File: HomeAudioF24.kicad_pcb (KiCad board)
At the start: 4 copper layers, 214 x 114 mm, 26 parts, among them U1 LF356M, U2 LF356M, U3 LF356M, U4 LF356M, U5 LF356M, U6 LF356M, U7 LF356M

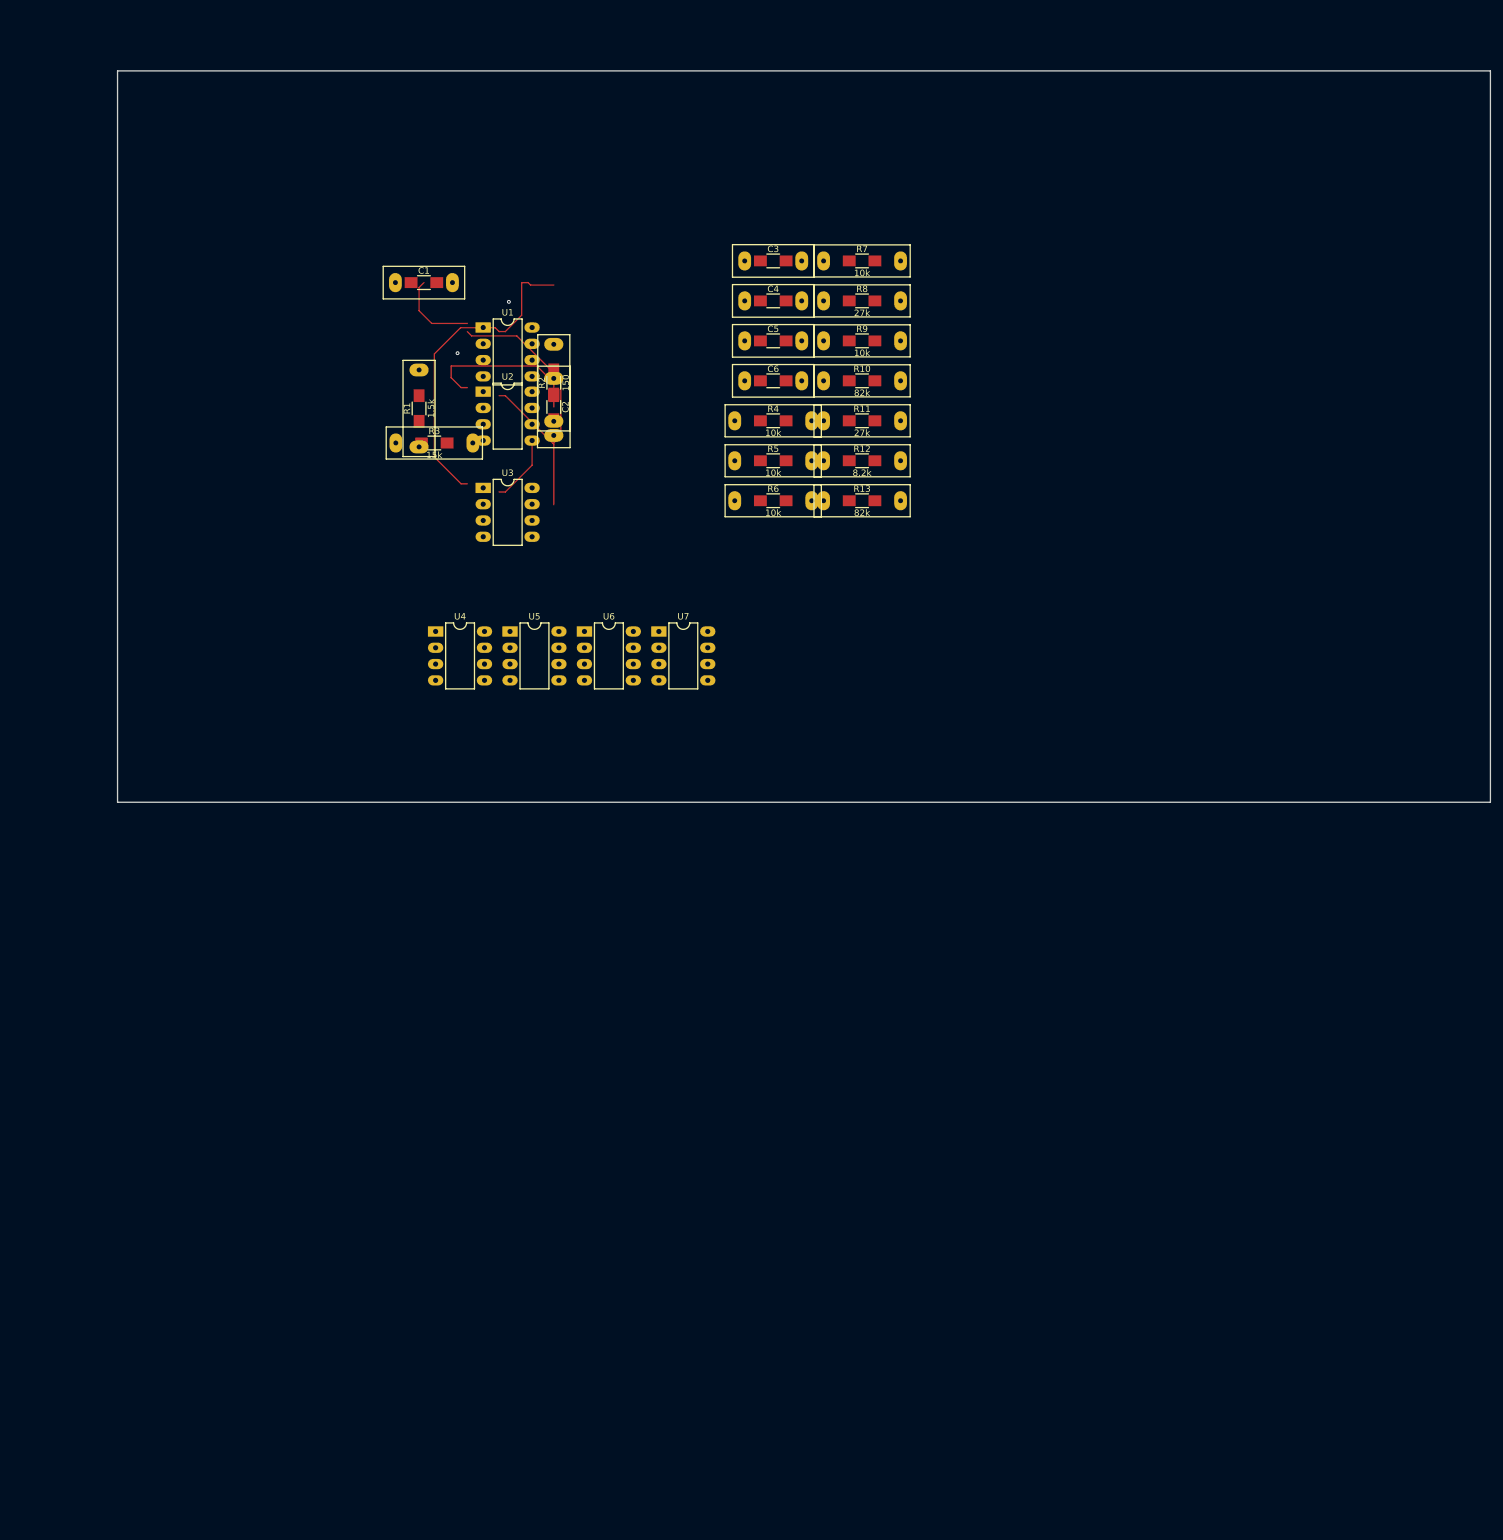
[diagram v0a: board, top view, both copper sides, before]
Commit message: First Major Revision
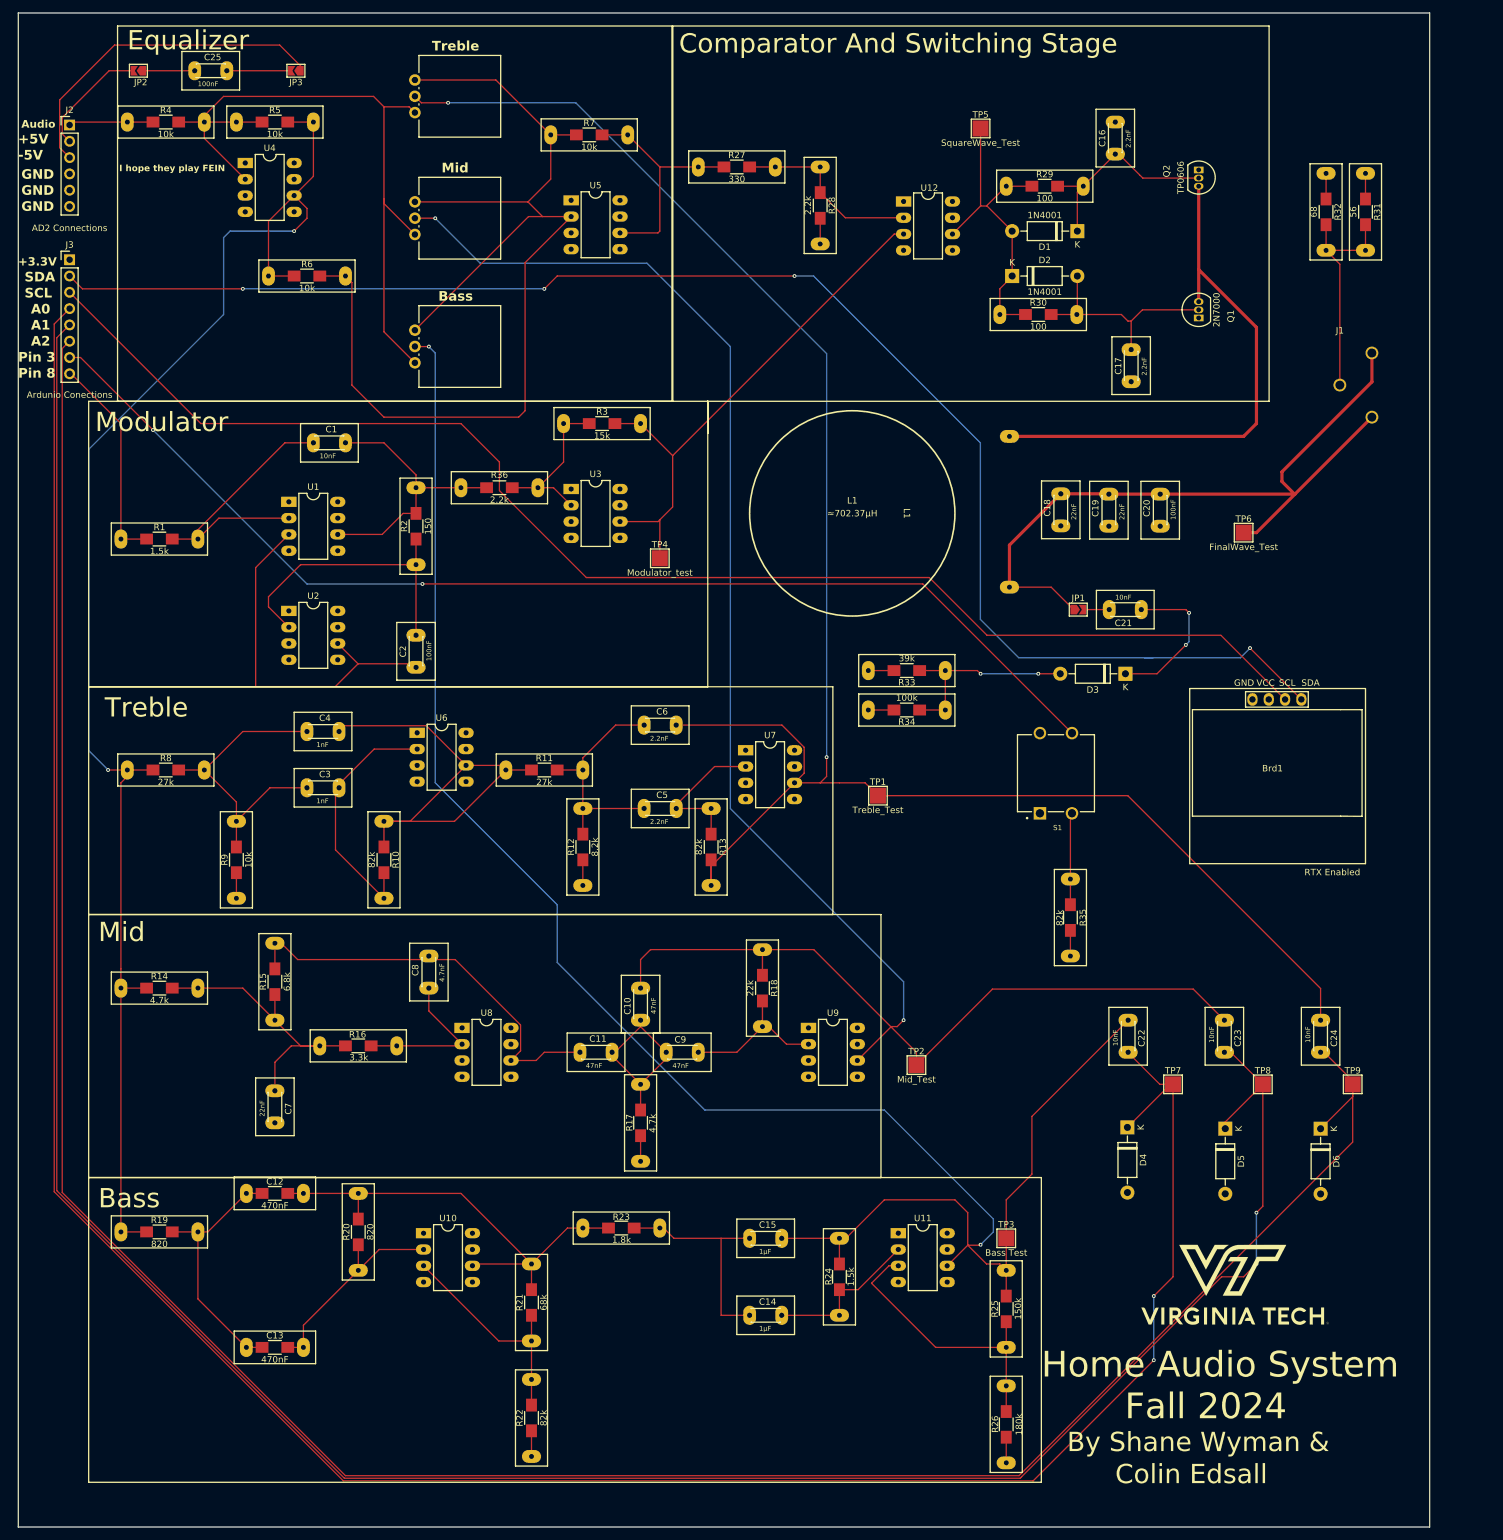
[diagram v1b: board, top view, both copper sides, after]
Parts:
- added Brd1: SSD1306, Display_New:128x64OLED SSD1306, F.Cu at (215.5, 142.6)
- added C10: 47nF, ColorOrgan:C_Disc_D4.3mm_W1.9mm_P5.00mm_Handsolder, F.Cu at (116.5, 177.0)
- added C11: 47nF, ColorOrgan:C_Disc_D4.3mm_W1.9mm_P5.00mm_Handsolder, F.Cu at (107.1, 187.0)
- added C12: 470nF, ColorOrgan:R_Combo, F.Cu at (59.5, 209.0)
- added C13: 470nF, ColorOrgan:R_Combo, F.Cu at (59.5, 233.0)
- added C14: 1μF, ColorOrgan:C_Disc_D4.3mm_W1.9mm_P5.00mm_Handsolder, F.Cu at (133.5, 228.0)
- added C15: 1μF, ColorOrgan:C_Disc_D4.3mm_W1.9mm_P5.00mm_Handsolder, F.Cu at (133.5, 216.0)
- added C16: 2.2nF, ColorOrgan:C_Disc_D4.3mm_W1.9mm_P5.00mm_Handsolder, F.Cu at (190.5, 42.0)
- added C17: 2.2nF, ColorOrgan:C_Disc_D4.3mm_W1.9mm_P5.00mm_Handsolder, F.Cu at (193.0, 77.4)
- added C18: 22nF, ColorOrgan:C_Disc_D4.3mm_W1.9mm_P5.00mm_Handsolder, F.Cu at (182.0, 104.9)
- added C19: 22nF, ColorOrgan:C_Disc_D4.3mm_W1.9mm_P5.00mm_Handsolder, F.Cu at (189.5, 105.0)
- added C20: 100nF, ColorOrgan:C_Disc_D4.3mm_W1.9mm_P5.00mm_Handsolder, F.Cu at (197.5, 105.0)
- added C21: 10nF, ColorOrgan:C_Disc_D4.3mm_W1.9mm_P5.00mm_Handsolder, F.Cu at (194.6, 118.0)
- added C22: 10nF, ColorOrgan:C_Disc_D4.3mm_W1.9mm_P5.00mm_Handsolder, F.Cu at (192.5, 182.0)
- added C23: 10nF, ColorOrgan:C_Disc_D4.3mm_W1.9mm_P5.00mm_Handsolder, F.Cu at (207.5, 182.0)
- added C24: 10nF, ColorOrgan:C_Disc_D4.3mm_W1.9mm_P5.00mm_Handsolder, F.Cu at (222.5, 182.0)
- added C25: 100nF, ColorOrgan:C_Disc_D4.3mm_W1.9mm_P5.00mm_Handsolder, F.Cu at (47.0, 34.0)
- added C7: 22nF, ColorOrgan:C_Disc_D4.3mm_W1.9mm_P5.00mm_Handsolder, F.Cu at (59.5, 193.0)
- added C8: 4.7nF, ColorOrgan:C_Disc_D4.3mm_W1.9mm_P5.00mm_Handsolder, F.Cu at (83.5, 177.0)
- added C9: 47nF, ColorOrgan:C_Disc_D4.3mm_W1.9mm_P5.00mm_Handsolder, F.Cu at (125.5, 187.0)
- added D1: 1N4001, Diode_THT:D_DO-41_SOD81_P10.16mm_Horizontal, F.Cu at (184.6, 59.0)
- added D2: 1N4001, Diode_THT:D_DO-41_SOD81_P10.16mm_Horizontal, F.Cu at (174.4, 66.0)
- added D3: 1N5817, Diode_THT:D_DO-41_SOD81_P10.16mm_Horizontal, F.Cu at (192.1, 128.0)
- added D4: 1N4001, Diode_THT:D_DO-41_SOD81_P10.16mm_Horizontal, F.Cu at (192.4, 198.7)
- added D5: 1N4001, Diode_THT:D_DO-41_SOD81_P10.16mm_Horizontal, F.Cu at (207.7, 198.9)
- added D6: 1N4001, Diode_THT:D_DO-41_SOD81_P10.16mm_Horizontal, F.Cu at (222.5, 198.9)
- added G***: LOGO, 4PinButton:vtSilkscreenFootPrint, F.Cu at (209.2, 223.2)
- added J1: AudioJack2_Ground, ColorOrgan:Jack_3.5mm_Ground_RightAngle, F.Cu at (225.5, 83.0)
- added J2: AD2 Connections, Connector_PinHeader_2.54mm:PinHeader_1x06_P2.54mm_Vertical, F.Cu at (27.5, 42.4)
- added J3: Ardunio Conections, Connector_PinHeader_2.54mm:PinHeader_1x08_P2.54mm_Vertical, F.Cu at (27.5, 63.4)
- added JP1: SolderJumper_2_Open, Jumper:SolderJumper-2_P1.3mm_Open_TrianglePad1.0x1.5mm, F.Cu at (184.8, 118.0)
- added JP2: SolderJumper_2_Open, Jumper:SolderJumper-2_P1.3mm_Open_TrianglePad1.0x1.5mm, F.Cu at (38.3, 34.0)
- added JP3: SolderJumper_2_Open, Jumper:SolderJumper-2_P1.3mm_Open_TrianglePad1.0x1.5mm, F.Cu at (62.8, 34.0)
- added L1: ≈702.37μH, ColorOrgan:InductorCore, F.Cu at (149.5, 103.0)
- added Q1: 2N7000, Package_TO_SOT_THT:TO-92_Inline, F.Cu at (203.5, 72.5)
- added Q2: TP0606, Package_TO_SOT_THT:TO-92L_Inline, F.Cu at (203.5, 49.4)
- added R14: 4.7k, ColorOrgan:1_2W Res + 1206, F.Cu at (41.5, 177.0)
- added R15: 6.8k, ColorOrgan:1_2W Res + 1206, F.Cu at (59.5, 176.0)
- added R16: 3.3k, ColorOrgan:1_2W Res + 1206, F.Cu at (72.5, 186.0)
- added R17: 4.7k, ColorOrgan:1_2W Res + 1206, F.Cu at (116.5, 198.0)
- added R18: 22k, ColorOrgan:1_2W Res + 1206, F.Cu at (135.5, 177.0)
- added R19: 820, ColorOrgan:1_2W Res + 1206, F.Cu at (41.5, 215.0)
- added R20: 820, ColorOrgan:1_2W Res + 1206, F.Cu at (72.5, 215.0)
- added R21: 68k, ColorOrgan:1_2W Res + 1206, F.Cu at (99.5, 226.0)
- added R22: 82k, ColorOrgan:1_2W Res + 1206, F.Cu at (99.5, 244.0)
- added R23: 1.8k, ColorOrgan:1_2W Res + 1206, F.Cu at (113.5, 214.4)
- added R24: 1.5k, ColorOrgan:1_2W Res + 1206, F.Cu at (147.5, 222.0)
- added R25: 150k, ColorOrgan:1_2W Res + 1206, F.Cu at (173.5, 227.0)
- added R26: 180k, ColorOrgan:1_2W Res + 1206, F.Cu at (173.5, 245.0)
- added R27: 330, ColorOrgan:1_2W Res + 1206, F.Cu at (131.5, 49.0)
- added R28: 2.2k, ColorOrgan:1_2W Res + 1206, F.Cu at (144.5, 55.0)
- added R29: 100, ColorOrgan:1_2W Res + 1206, F.Cu at (179.5, 52.0)
- added R30: 100, ColorOrgan:1_2W Res + 1206, F.Cu at (178.5, 72.0)
- added R31: 56, ColorOrgan:1_2W Res + 1206, F.Cu at (229.5, 56.0)
- added R32: 68, ColorOrgan:1_2W Res + 1206, F.Cu at (223.4, 56.0)
- added R33: 39k, ColorOrgan:1_2W Res + 1206, F.Cu at (158.0, 127.5)
- added R34: 100k, ColorOrgan:1_2W Res + 1206, F.Cu at (158.0, 133.6)
- added R35: 82k, ColorOrgan:1_2W Res + 1206, F.Cu at (183.5, 166.0)
- added R36: 2.2k, ColorOrgan:1_2W Res + 1206, F.Cu at (94.5, 99.0)
- added RV1: R_Potentiometer, Potentiometer_THT:Potentiometer_Vishay_148-149_Single_Vertical, F.Cu at (81.4, 40.5)
- added RV2: R_Potentiometer, Potentiometer_THT:Potentiometer_Vishay_148-149_Single_Vertical, F.Cu at (81.4, 59.5)
- added RV3: R_Potentiometer, Potentiometer_THT:Potentiometer_Vishay_148-149_Single_Vertical, F.Cu at (81.4, 79.5)
- added S1: VS-1213-67-160GF, 4PinButton:SW_VS-1213-67-160GF, F.Cu at (181.3, 143.5)
- added TP1: Treble_Test, TestPoint:TestPoint_Pad_2.5x2.5mm, F.Cu at (153.5, 147.0)
- added TP2: Mid_Test, TestPoint:TestPoint_Pad_2.5x2.5mm, F.Cu at (159.5, 189.0)
- added TP3: Bass Test, TestPoint:TestPoint_Pad_2.5x2.5mm, F.Cu at (173.5, 216.0)
- added TP4: Modulator_test, TestPoint:TestPoint_Pad_2.5x2.5mm, F.Cu at (119.5, 110.0)
- added TP5: SquareWave_Test, TestPoint:TestPoint_Pad_2.5x2.5mm, F.Cu at (169.5, 43.0)
- added TP6: FinalWave_Test, TestPoint:TestPoint_Pad_2.5x2.5mm, F.Cu at (210.5, 106.0)
- added TP7: A0_Test, TestPoint:TestPoint_Pad_2.5x2.5mm, F.Cu at (199.5, 192.0)
- added TP8: A1_Test, TestPoint:TestPoint_Pad_2.5x2.5mm, F.Cu at (213.5, 192.0)
- added TP9: A2_Test, TestPoint:TestPoint_Pad_2.5x2.5mm, F.Cu at (227.5, 192.0)
- added U10: LF356M, Package_DIP:DIP-8_W7.62mm_LongPads, F.Cu at (82.7, 215.2)
- added U11: LF356M, Package_DIP:DIP-8_W7.62mm_LongPads, F.Cu at (156.7, 215.2)
- added U12: LF356M, Package_DIP:DIP-8_W7.62mm_LongPads, F.Cu at (157.5, 54.4)
- added U8: LF356M, Package_DIP:DIP-8_W7.62mm_LongPads, F.Cu at (88.7, 183.2)
- added U9: LF356M, Package_DIP:DIP-8_W7.62mm_LongPads, F.Cu at (142.7, 183.2)
- C1: value .01μ -> 10nF; footprint ColorOrgan:R_Combo -> ColorOrgan:C_Disc_D4.3mm_W1.9mm_P5.00mm_Handsolder
- C2: value .1μ -> 100nF; footprint ColorOrgan:R_Combo -> ColorOrgan:C_Disc_D4.3mm_W1.9mm_P5.00mm_Handsolder
- C3, C4, C5, C6: footprint ColorOrgan:R_Combo -> ColorOrgan:C_Disc_D4.3mm_W1.9mm_P5.00mm_Handsolder
- moved R8 130.9 mm to (42.5, 143.0)
- moved R9 126.7 mm to (53.5, 157.0), turned to 90 degrees
- moved C3 109.7 mm to (64.5, 145.7)
- moved R4 105.5 mm to (42.5, 42.0)
- moved R10 105.5 mm to (76.5, 157.0), turned to -90 degrees
- moved C4 98.9 mm to (64.5, 137.0)
- moved R5 93.9 mm to (59.5, 42.0)
- moved R6 80.7 mm to (64.5, 66.0)
- moved U4 78.8 mm to (54.9, 48.4)
- moved C5 75.6 mm to (117.1, 149.0)
- moved R12 74.3 mm to (107.5, 155.0), turned to 90 degrees
- moved R11 73.6 mm to (101.5, 143.0)
- moved U5 67.9 mm to (105.7, 54.2)
- moved R13 58.9 mm to (127.5, 155.0), turned to -90 degrees
- moved C6 57.3 mm to (117.1, 136.0)
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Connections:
- R3 pad 1: Net-(U1-OUT) -> Net-(U3--IN)
- U3 pad 2: Net-(U1-OUT) -> Net-(U3--IN)
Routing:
- net A1: track 0.00 -> 401.2 mm, vias 0 -> 2
- net A0: track 0.00 -> 399.8 mm, vias 0 -> 2
- net A2: track 0.00 -> 399.8 mm
- net Bass_Out: track 0.00 -> 303.8 mm, vias 0 -> 2
- net Treble_Out: track 0.00 -> 302.0 mm, vias 0 -> 2
- net Mid_Out: track 0.00 -> 299.1 mm, vias 0 -> 2
- net SDA: track 0.00 -> 239.8 mm, vias 0 -> 4
- net Bass_In: track 0.00 -> 233.9 mm, vias 0 -> 2
- net SCL: track 0.00 -> 218.4 mm
- net Button_Pin: track 0.00 -> 180.5 mm, vias 0 -> 2
- net Net-(U5--IN): track 0.00 -> 177.3 mm
- net Net-(JP1-A): track 0.00 -> 123.7 mm
- net Net-(U4--IN): track 0.00 -> 110.1 mm
- net Net-(Q1-D): track 0.00 -> 85.1 mm
- net Modulator_Out: track 0.00 -> 84.5 mm
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- added copper zone on In2.Cu, net +3.3V
- added copper zone on In2.Cu, net -5V
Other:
- board size 214 x 114 mm -> 220 x 236 mm
- board text added: "+3.3V"
- board text added: "+5V"
- board text added: "-5V"
- board text added: "A0"
- board text added: "A1"
- board text added: "A2"
- board text added: "Audio"
- board text added: "Bass"
- board text added: "By Shane Wyman &"
- board text added: "Colin Edsall"
- board text added: "Comparator And Switching Stage"
- board text added: "Equalizer"
- board text added: "Fall 2024"
- board text added: "GND"
- board text added: "Home Audio System"
- board text added: "I hope they play FEIN"
- board text added: "Mid"
- board text added: "Modulator"
- board text added: "Pin 3"
- board text added: "Pin 8"
- board text added: "RTX Enabled"
- board text added: "SCL"
- board text added: "SDA"
- board text added: "Treble"
